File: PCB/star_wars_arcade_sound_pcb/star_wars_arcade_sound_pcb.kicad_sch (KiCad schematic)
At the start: 0 parts

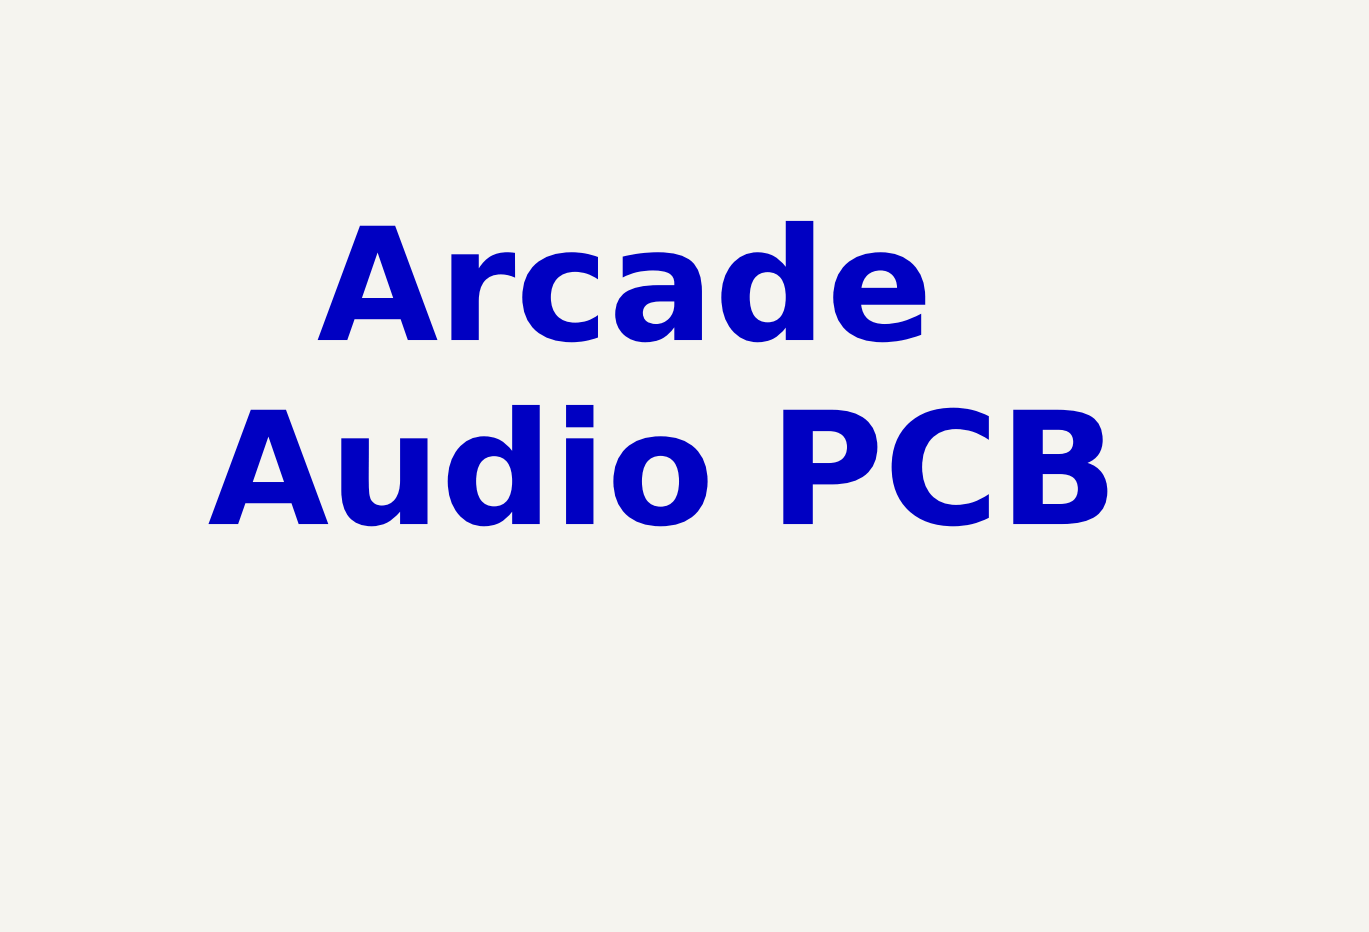
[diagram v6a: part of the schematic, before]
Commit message: Updated schematic
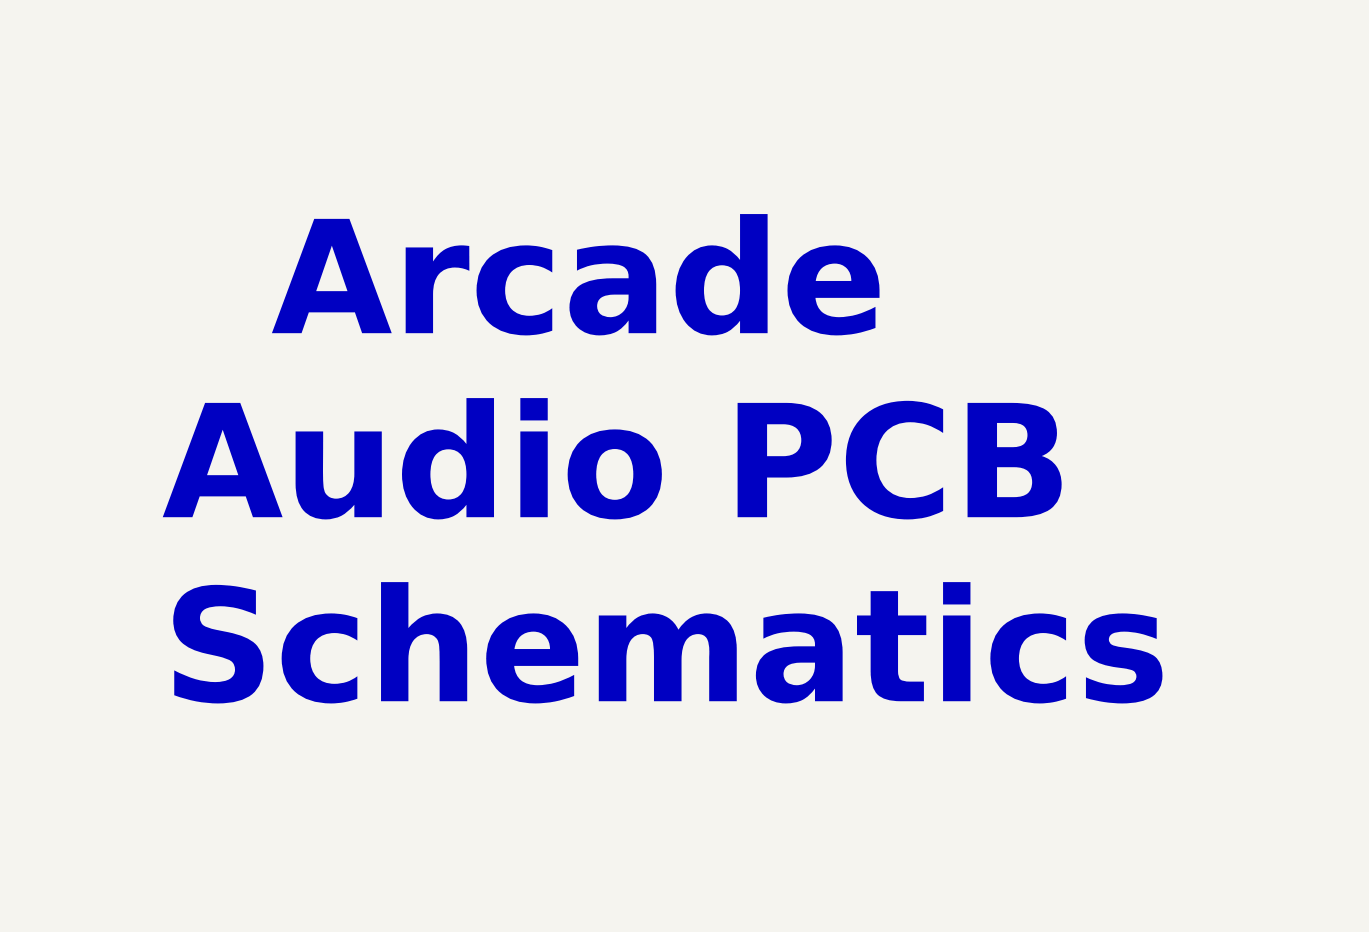
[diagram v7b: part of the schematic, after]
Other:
- note added: "Arcade Audio PCB Schematics"
- note removed: "Arcade Audio PCB"
